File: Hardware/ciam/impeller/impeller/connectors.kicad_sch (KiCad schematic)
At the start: 22 parts, among them J12 Micro-Fit_2x2P, J14 PLS-5, J29 USBA-1J, Q1 BSS138, Q2 BSS138, U4 B0505MT-1WR4, U4 USBLC6-2SC6, U46 HCPL-0630, U47 LDL1117S33R

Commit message: updated bom
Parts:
- C14, C63: Человекопонятное название (none) -> Конденсатор 4.7мкФ
- C16: Человекопонятное название (none) -> Конденсатор 10мкФ
- C20, C59, C62: Человекопонятное название (none) -> Конденсатор 100нФ
- D3: Человекопонятное название (none) -> Диод Шоттки
- J12: Человекопонятное название (none) -> Разъем Micro-Fit 2x2 М
- J14: Человекопонятное название (none) -> Вилка штыревая 1x5
- J29: Человекопонятное название (none) -> Разъем USB A
- Q1, Q2: Человекопонятное название (none) -> Транзистор полевой n типа
- R100, R101, R102, R99: Человекопонятное название (none) -> Резистор 10k Ом
- R51: Человекопонятное название (none) -> Резистор 220 Ом
- U4: Человекопонятное название (none) -> DC/DC преобразователь
- U4: Человекопонятное название (none) -> Защита интерфейса USB от электростатических разрядов
- U46: Человекопонятное название (none) -> Оптопара двухканальная с логическими уровнями на выходе
- U47: Человекопонятное название (none) -> LDO-стабилизатор напряжения
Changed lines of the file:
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@@
+      (effects (font (size 1.27 1.27)) hide)
+    )
+    (property "Человекопонятное название" "Конденсатор 100нФ" (at 100.33 148.59 0)
       (effects (font (size 1.27 1.27)) hide)
     )
@@
     )
     (property "Цена" "5" (at 66.04 118.745 0)
+      (effects (font (size 1.27 1.27)) hide)
+    )
+    (property "Человекопонятное название" "Резистор 220 Ом" (at 66.04 118.745 0)
       (effects (font (size 1.27 1.27)) hide)
     )
@@
     )
     (property "Цена" "" (at 77.47 111.125 0)
+      (effects (font (size 1.27 1.27)) hide)
+    )
+    (property "Человекопонятное название" "Оптопара двухканальная с логическими уровнями на выходе" (at 77.47 111.125 0)
       (effects (font (size 1.27 1.27)) hide)
     )
@@
       (effects (font (size 1.27 1.27)) hide)
     )
+    (property "Человекопонятное название" "Конденсатор 10мкФ" (at 72.39 147.32 0)
+      (effects (font (size 1.27 1.27)) hide)
+    )
     (pin "1")
     (pin "2")
@@
       (effects (font (size 1.27 1.27)) hide)
     )
+    (property "Человекопонятное название" "Конденсатор 4.7мкФ" (at 135.255 148.59 0)
+      (effects (font (size 1.27 1.27)) hide)
+    )
     (pin "1")
     (pin "2")
@@
       (effects (font (size 1.27 1.27)) hide)
     )
+    (property "Человекопонятное название" "LDO-стабилизатор напряжения" (at 116.205 143.51 0)
+      (effects (font (size 1.27 1.27)) hide)
+    )
     (pin "1")
     (pin "2")
@@
       (effects (font (size 1.27 1.27)) hide)
     )
+    (property "Человекопонятное название" "Резистор 10k Ом" (at 127.635 113.665 0)
+      (effects (font (size 1.27 1.27)) hide)
+    )
     (pin "1")
     (pin "2")
@@
       (effects (font (size 1.27 1.27)) hide)
     )
+    (property "Человекопонятное название" "Разъем Micro-Fit 2x2 М" (at 151.13 106.045 0)
+      (effects (font (size 1.27 1.27)) hide)
+    )
     (pin "1")
     (pin "2")
@@
     )
     (property "Цена" "5" (at 127.635 100.965 0)
+      (effects (font (size 1.27 1.27)) hide)
+    )
+    (property "Человекопонятное название" "Резистор 10k Ом" (at 127.635 100.965 0)
       (effects (font (size 1.27 1.27)) hide)
     )
@@
       (effects (font (size 1.27 1.27)) hide)
     )
+    (property "Человекопонятное название" "Разъем USB A" (at 43.18 52.07 0)
+      (effects (font (size 1.27 1.27)) hide)
+    )
     (pin "1")
     (pin "2")
@@
       (effects (font (size 1.27 1.27)) hide)
     )
+    (property "Человекопонятное название" "Резистор 220 Ом" (at 66.04 103.505 0)
+      (effects (font (size 1.27 1.27)) hide)
+    )
     (pin "1")
     (pin "2")
@@
       (effects (font (size 1.27 1.27)) hide)
     )
+    (property "Человекопонятное название" "Транзистор полевой n типа" (at 121.285 116.205 0)
+      (effects (font (size 1.27 1.27)) hide)
+    )
     (pin "1")
     (pin "2")
@@
     )
     (property "Цена" "120" (at 51.435 146.05 0)
+      (effects (font (size 1.27 1.27)) hide)
+    )
+    (property "Человекопонятное название" "DC/DC преобразователь" (at 51.435 146.05 0)
       (effects (font (size 1.27 1.27)) hide)
     )
@@
       (effects (font (size 1.27 1.27)) hide)
     )
+    (property "Человекопонятное название" "Конденсатор 100нФ" (at 33.655 52.705 0)
+      (effects (font (size 1.27 1.27)) hide)
+    )
     (pin "1")
     (pin "2")
@@
       (effects (font (size 1.27 1.27)) hide)
     )
+    (property "Человекопонятное название" "Вилка штыревая 1x5" (at 155.575 45.085 0)
+      (effects (font (size 1.27 1.27)) hide)
+    )
     (pin "1")
     (pin "2")
@@
       (effects (font (size 1.27 1.27)) hide)
     )
+    (property "Человекопонятное название" "Конденсатор 4.7мкФ" (at 35.56 147.32 0)
+      (effects (font (size 1.27 1.27)) hide)
+    )
     (pin "1")
     (pin "2")
@@
       (effects (font (size 1.27 1.27)) hide)
     )
+    (property "Человекопонятное название" "Транзистор полевой n типа" (at 121.285 103.505 0)
+      (effects (font (size 1.27 1.27)) hide)
+    )
     (pin "1")
     (pin "2")
@@
     )
     (property "Цена" "25" (at 92.075 53.34 0)
+      (effects (font (size 1.27 1.27)) hide)
+    )
+    (property "Человекопонятное название" "Защита интерфейса USB от электростатических разрядов" (at 92.075 53.34 0)
       (effects (font (size 1.27 1.27)) hide)
     )
@@
       (effects (font (size 1.27 1.27)) hide)
     )
+    (property "Человекопонятное название" "Диод Шоттки" (at 57.785 46.99 0)
+      (effects (font (size 1.27 1.27)) hide)
+    )
     (pin "1")
     (pin "2")
@@
       (effects (font (size 1.27 1.27)) hide)
     )
+    (property "Человекопонятное название" "Резистор 10k Ом" (at 114.935 113.665 0)
+      (effects (font (size 1.27 1.27)) hide)
+    )
     (pin "1")
     (pin "2")
@@
     )
     (property "Цена" "5" (at 114.935 100.965 0)
+      (effects (font (size 1.27 1.27)) hide)
+    )
+    (property "Человекопонятное название" "Резистор 10k Ом" (at 114.935 100.965 0)
       (effects (font (size 1.27 1.27)) hide)
     )
@@
       (effects (font (size 1.27 1.27)) hide)
     )
+    (property "Человекопонятное название" "Конденсатор 100нФ" (at 85.725 100.965 0)
+      (effects (font (size 1.27 1.27)) hide)
+    )

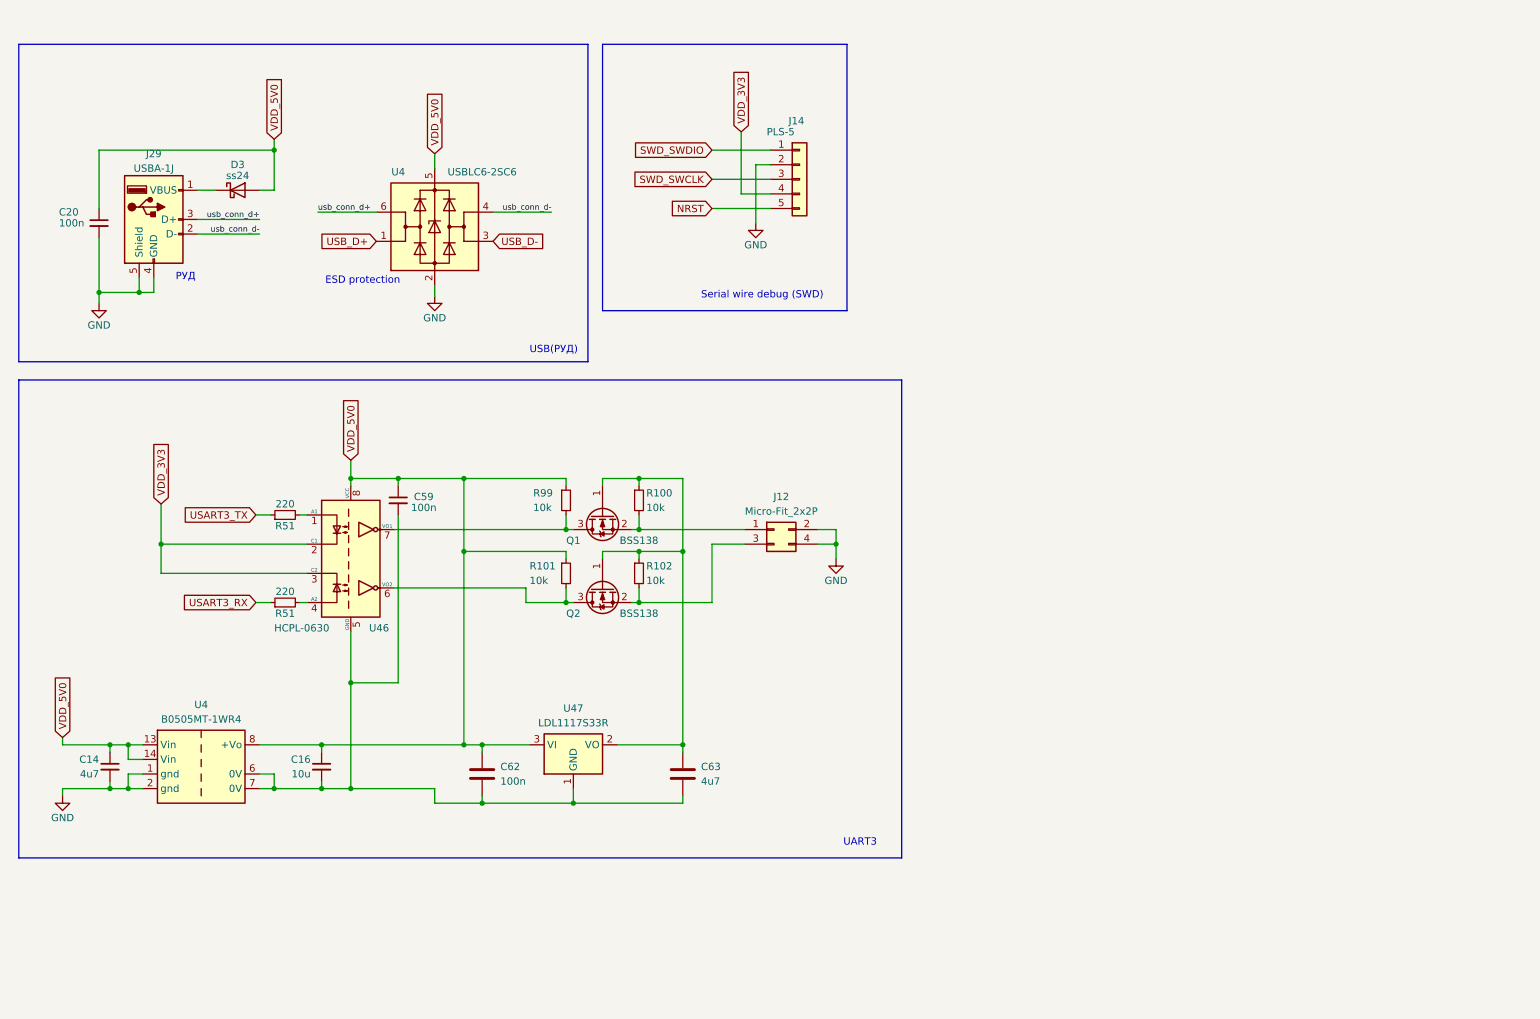
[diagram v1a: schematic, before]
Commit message: Updated CIAM project
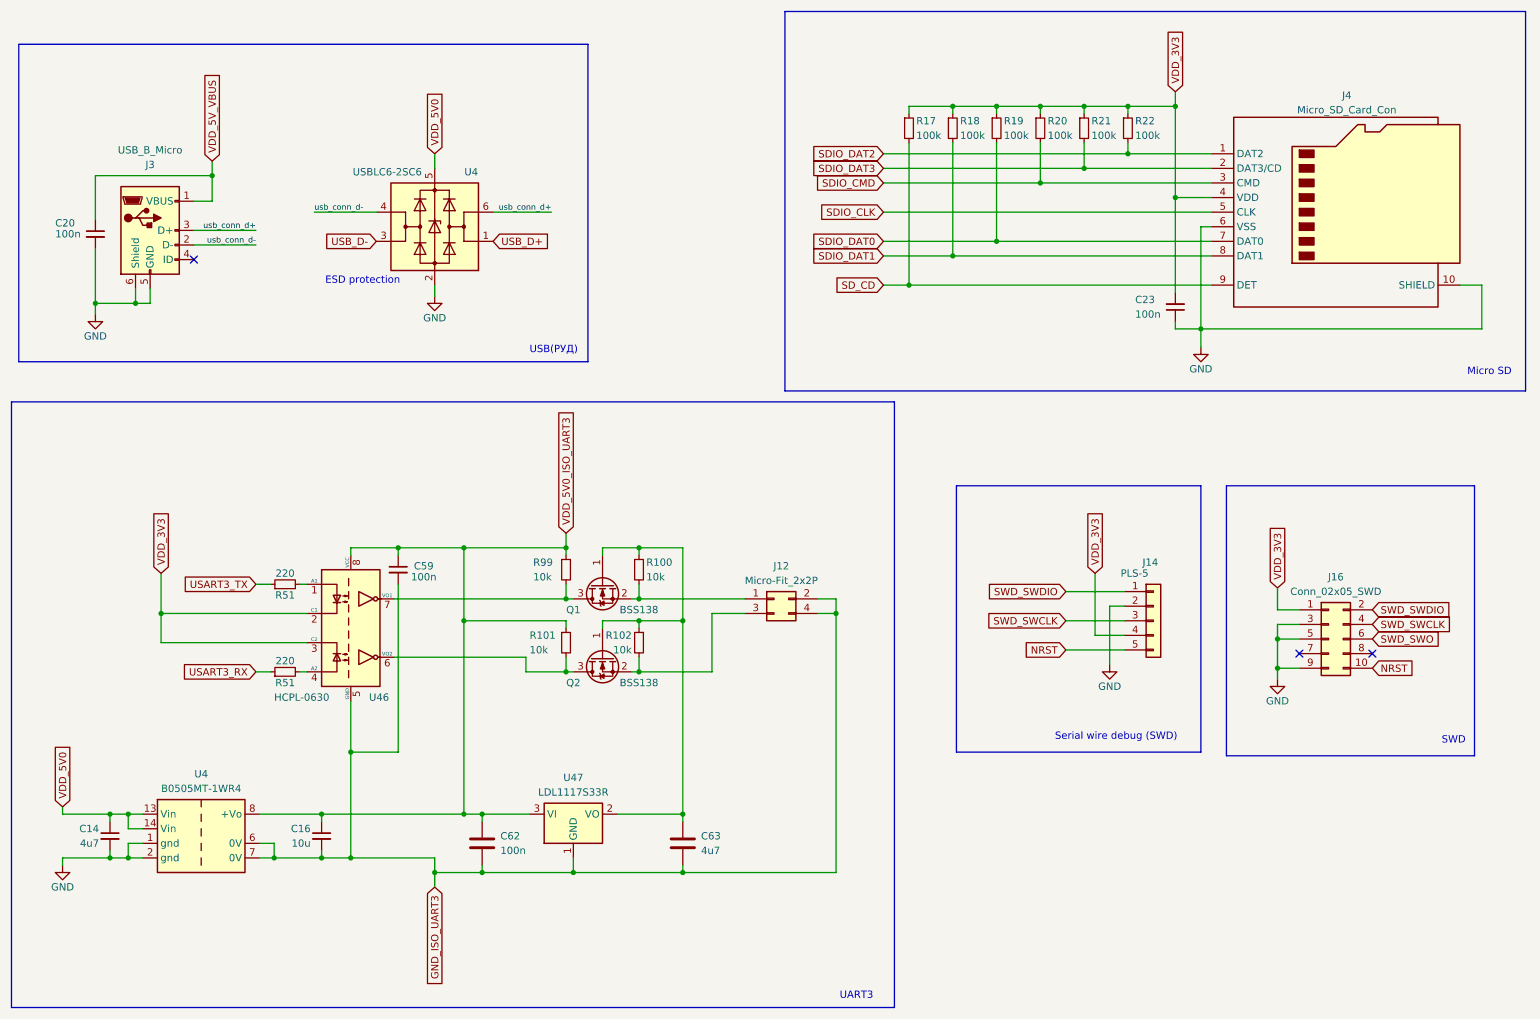
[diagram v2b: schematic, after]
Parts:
- removed D3: ss24, symbol Device:D_Schottky
- removed J29: USBA-1J, symbol Connector:USB_A
- added C23: 100n, Capacitor_SMD:C_0603_1608Metric, symbol Device:C_Small
- added J16: Conn_02x05_SWD, Connector_PinHeader_1.27mm:PinHeader_2x05_P1.27mm_Vertical, symbol Connector_Generic:Conn_02x05_Odd_Even
- added J3: USB_B_Micro, user_lib:U-F-M5DD-W-2-SUS, symbol Connector:USB_B_Micro
- added J4: Micro_SD_Card_Con, sd:TF01A, symbol Connector:Micro_SD_Card_Det1
- added R17, R18, R19, R20, R21, R22: 100k, Resistor_SMD:R_0603_1608Metric, symbol Device:R_Small
- J12: footprint (none) -> Connector_Molex:Molex_Micro-Fit_3.0_43045-0400_2x02_P3.00mm_Horizontal; Ссылка https://www.chipdip.ru/product/sct3001wv-2x02p -> https://www.chipdip.ru/product/sct3001wr-2x02p
- J14: footprint (none) -> Connector_PinHeader_2.54mm:PinHeader_1x05_P2.54mm_Vertical
- U4: footprint (none) -> user_lib:B0505MT-1WR4
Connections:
- net GND: now also C23.1, J16.3 (Pin_3), J16.5 (Pin_5), J16.9 (Pin_9), J3.5 (GND), J3.6 (Shield), J4.10 (SHIELD), J4.6 (VSS); no longer J12.2 (Pin_2), J12.4 (Pin_4)
- net NRST: now also J16.10 (Pin_10)
- net SWD_SWCLK: now also J16.4 (Pin_4)
- net SWD_SWDIO: now also J16.2 (Pin_2)
- net VDD_3V3: now also C23.2, J16.1 (Pin_1), J4.4 (VDD), R17.1, R18.1, R19.1, R20.1, R21.1, R22.1
- net VDD_5V0: no longer C16.1, C20.1, C59.1, C62.1, R101.1, R99.1, U4.8 (+Vo), U46.8 (VCC), U47.3 (VI)
- net usb_conn_d+: now also J3.3 (D+)
- net usb_conn_d-: now also J3.2 (D-)
- net GND_ISO_UART3: now reaches C16.2, C59.2, C62.2, C63.2, U4.6 (0V), U4.7 (0V), U46.5 (GND), U47.1 (GND)
- net GND_ISO_UART3: now also J12.2 (Pin_2), J12.4 (Pin_4)
- new net SDIO_CLK: J4.5 (CLK)
- new net SDIO_CMD: J4.3 (CMD), R20.2
- new net SDIO_DAT0: J4.7 (DAT0), R19.2
- new net SDIO_DAT1: J4.8 (DAT1), R18.2
- new net SDIO_DAT2: J4.1 (DAT2), R22.2
- new net SDIO_DAT3: J4.2 (DAT3/CD), R21.2
- new net SD_CD: J4.9 (DET), R17.2
- new net SWD_SWO: J16.6 (Pin_6)
- new net VDD_5V0_ISO_UART3: C16.1, C59.1, C62.1, R101.1, R99.1, U4.8 (+Vo), U46.8 (VCC), U47.3 (VI)
- new net VDD_5V_VBUS: C20.1, J3.1 (VBUS)
- no-connect marks 0 -> 3
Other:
- note added: "Micro SD"
- note added: "SWD"
- note removed: "РУД"
- moved on the sheet: C14, C16, C59, C62, C63, J12, J14, Q1, Q2, R100, R101, R102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

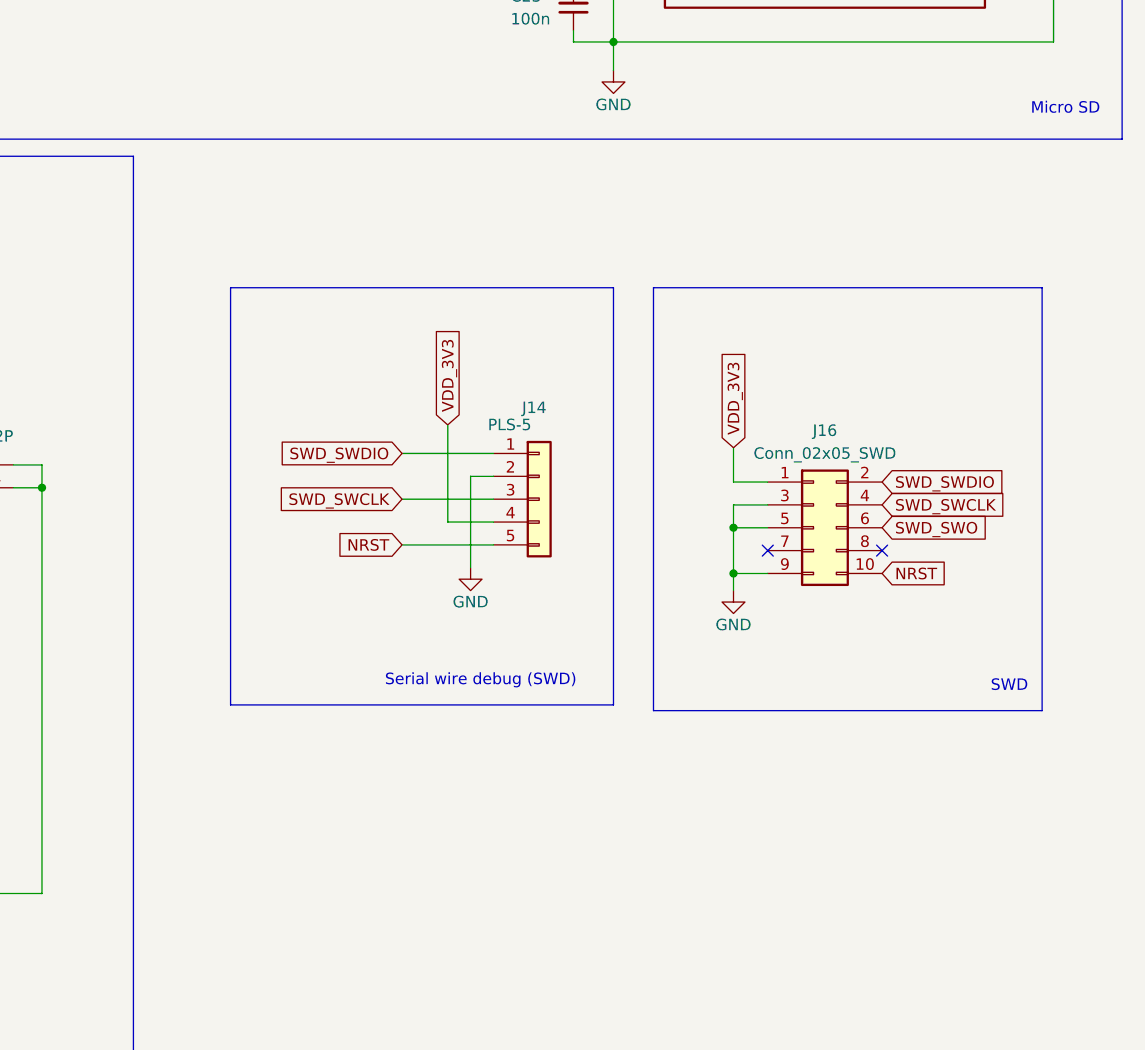
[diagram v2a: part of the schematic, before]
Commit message: added thrust lever
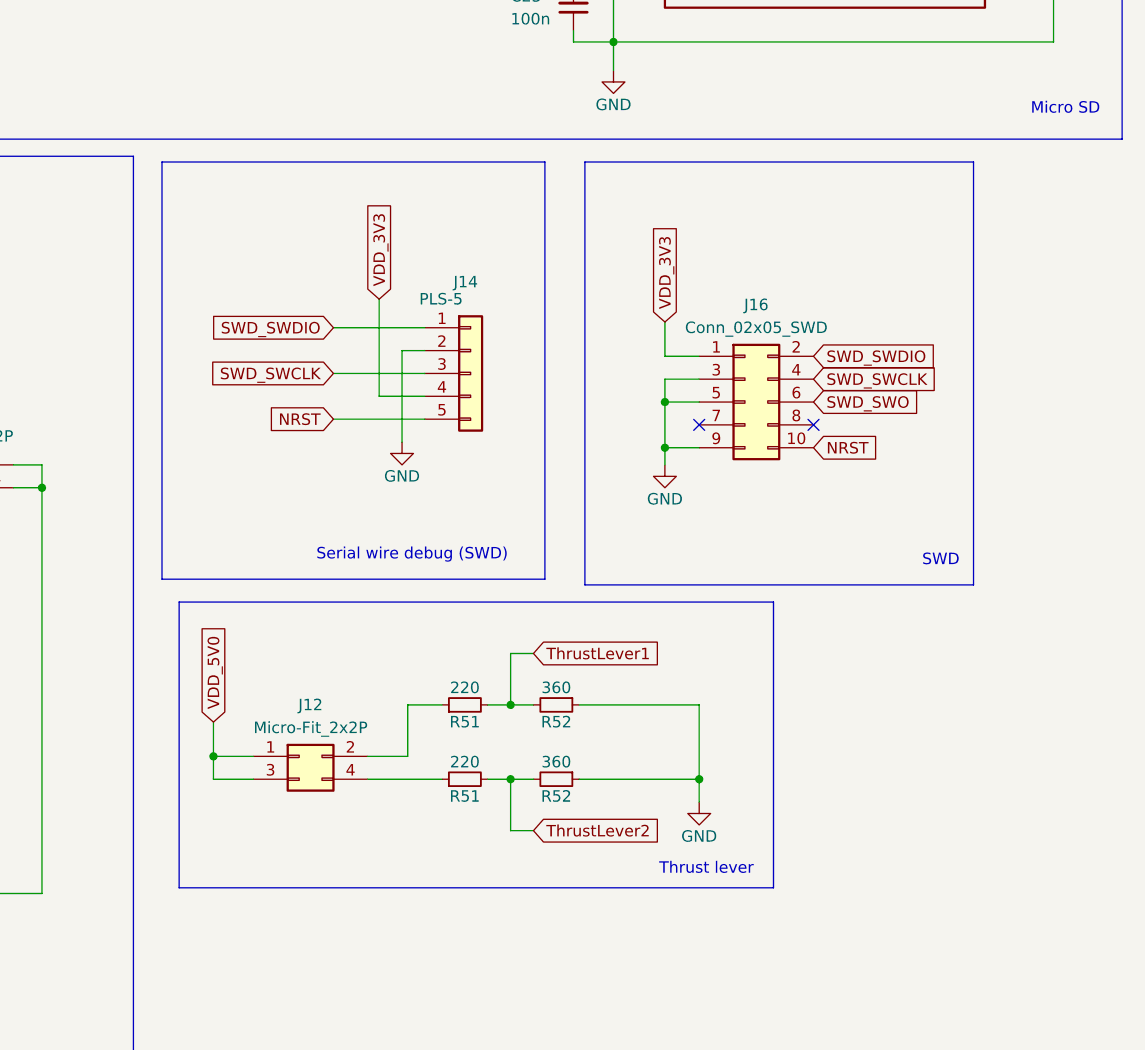
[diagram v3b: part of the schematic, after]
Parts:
- added J12: Micro-Fit_2x2P, Connector_Molex:Molex_Micro-Fit_3.0_43045-0400_2x02_P3.00mm_Horizontal, symbol Connector_Generic:Conn_02x02_Odd_Even
- added R51 (x2): 220, Resistor_SMD:R_0603_1608Metric, symbol Device:R_Small
- added R52 (x2): 360, Resistor_SMD:R_0603_1608Metric, symbol Device:R_Small
- R17, R18, R19, R20, R21, R22: Ссылка (none) -> https://www.chipdip.ru/product/0.1w-0603-100-kom-1; Цена (none) -> 5; Человекопонятное название (none) -> Резистор 100k Ом
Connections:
- net GND: now also R52.1, R52.1
- net VDD_5V0: now also J12.1 (Pin_1), J12.3 (Pin_3)
- new net: J12.2 (Pin_2), R51.1
- new net: J12.4 (Pin_4), R51.1
- new net ThrustLever1: R51.2, R52.2
- new net ThrustLever2: R51.2, R52.2
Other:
- note added: "Thrust lever"
- moved on the sheet: J14, J16
